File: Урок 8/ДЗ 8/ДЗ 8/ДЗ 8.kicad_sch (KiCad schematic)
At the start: 34 parts, among them K1 HONGFA_HFD2-0xx-x-L2-x, K2 HONGFA_HFD2-0xx-x-L2-x, SW1 SW_Push, SW2 SW_Push

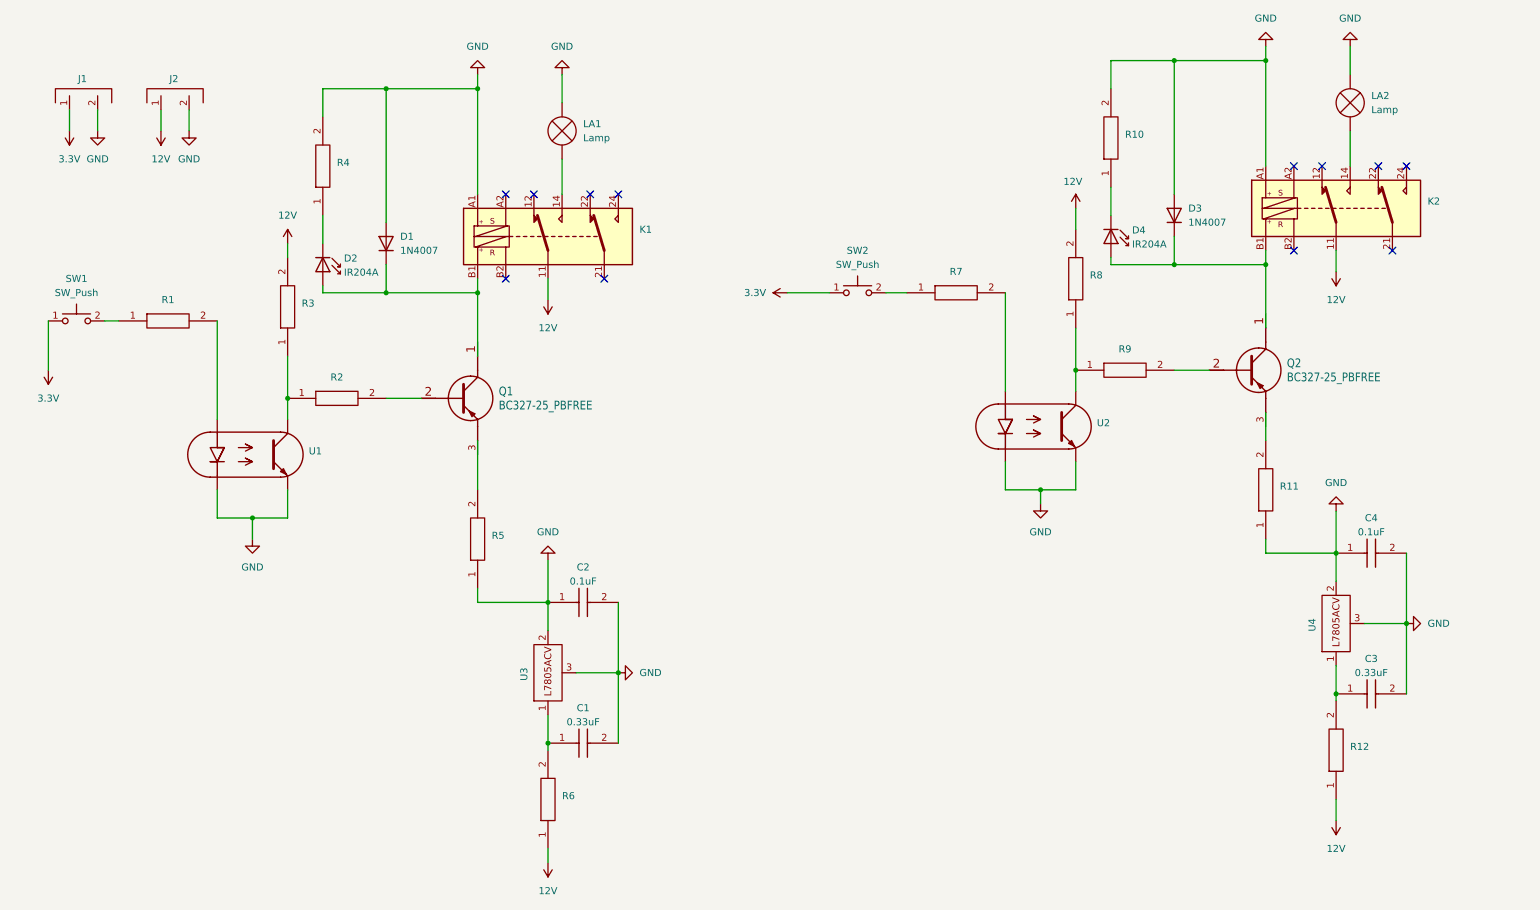
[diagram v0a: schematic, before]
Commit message: 1
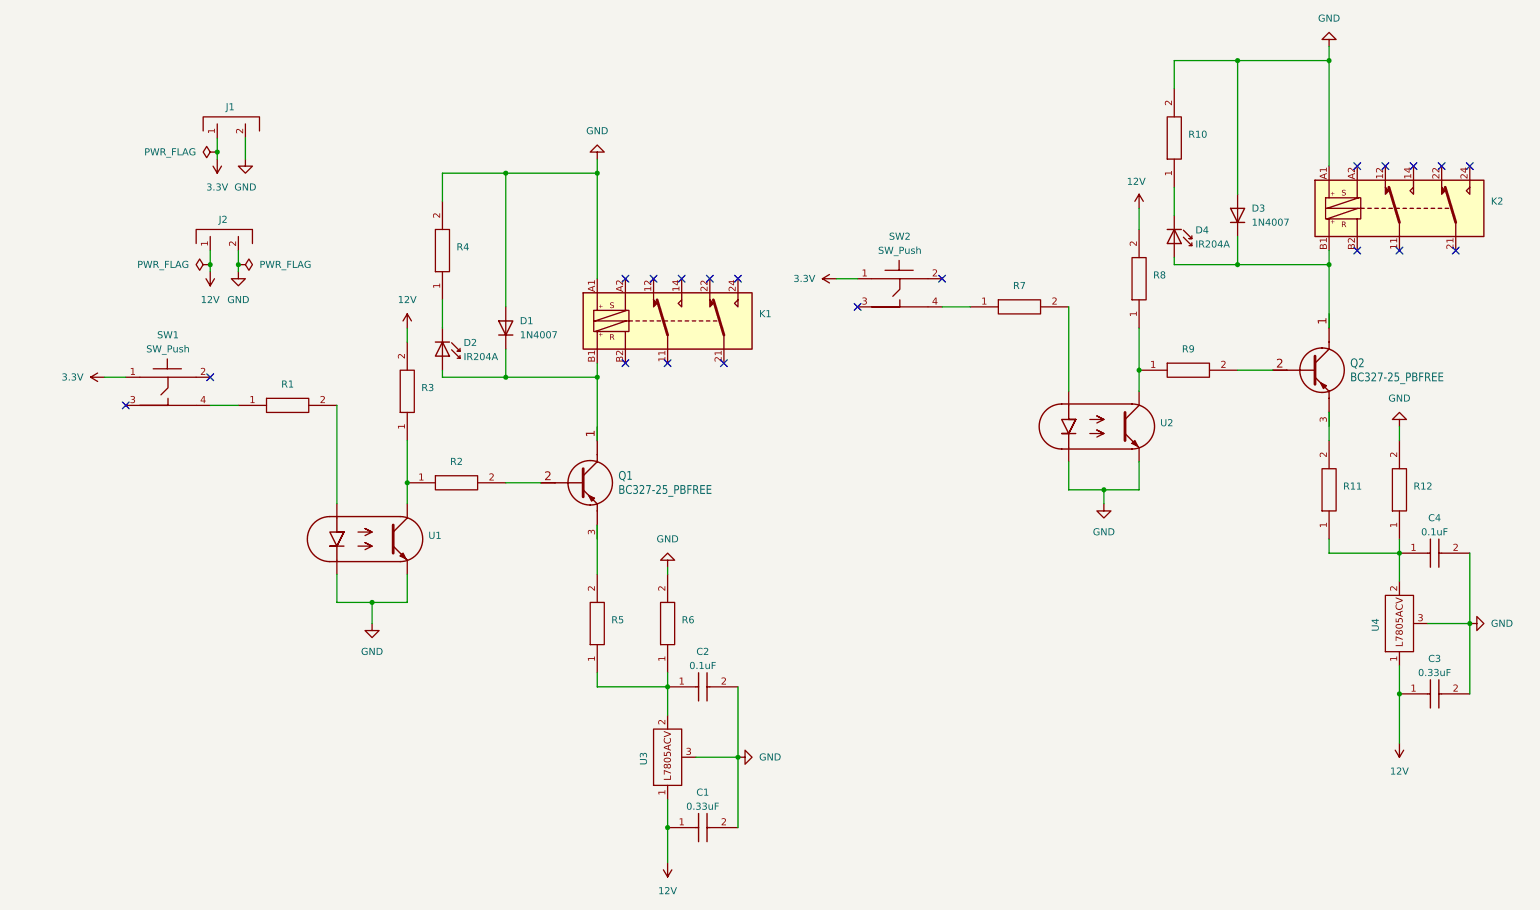
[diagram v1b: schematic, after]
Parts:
- removed LA1, LA2: Lamp, symbol Device:Lamp
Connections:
- net 12V: now also C1.1, C3.1, U3.1, U4.1; no longer K1.11, K2.11, R12.1, R6.1
- net GND: now also R12.2, R6.2; no longer C2.1, C4.1, R11.1, R5.1, U3.2, U4.2
- net at R1.1: now also SW1.4 (2); no longer SW1.2
- net at R7.1: now also SW2.4 (2); no longer SW2.2
- new net: C4.1, R11.1, R12.1, U4.2
- new net: C2.1, R5.1, R6.1, U3.2
- no-connect marks 12 -> 20
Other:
- moved on the sheet: C1, C2, C3, C4, D1, D2, D3, D4, J1, J2, K1, K2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

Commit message: 1
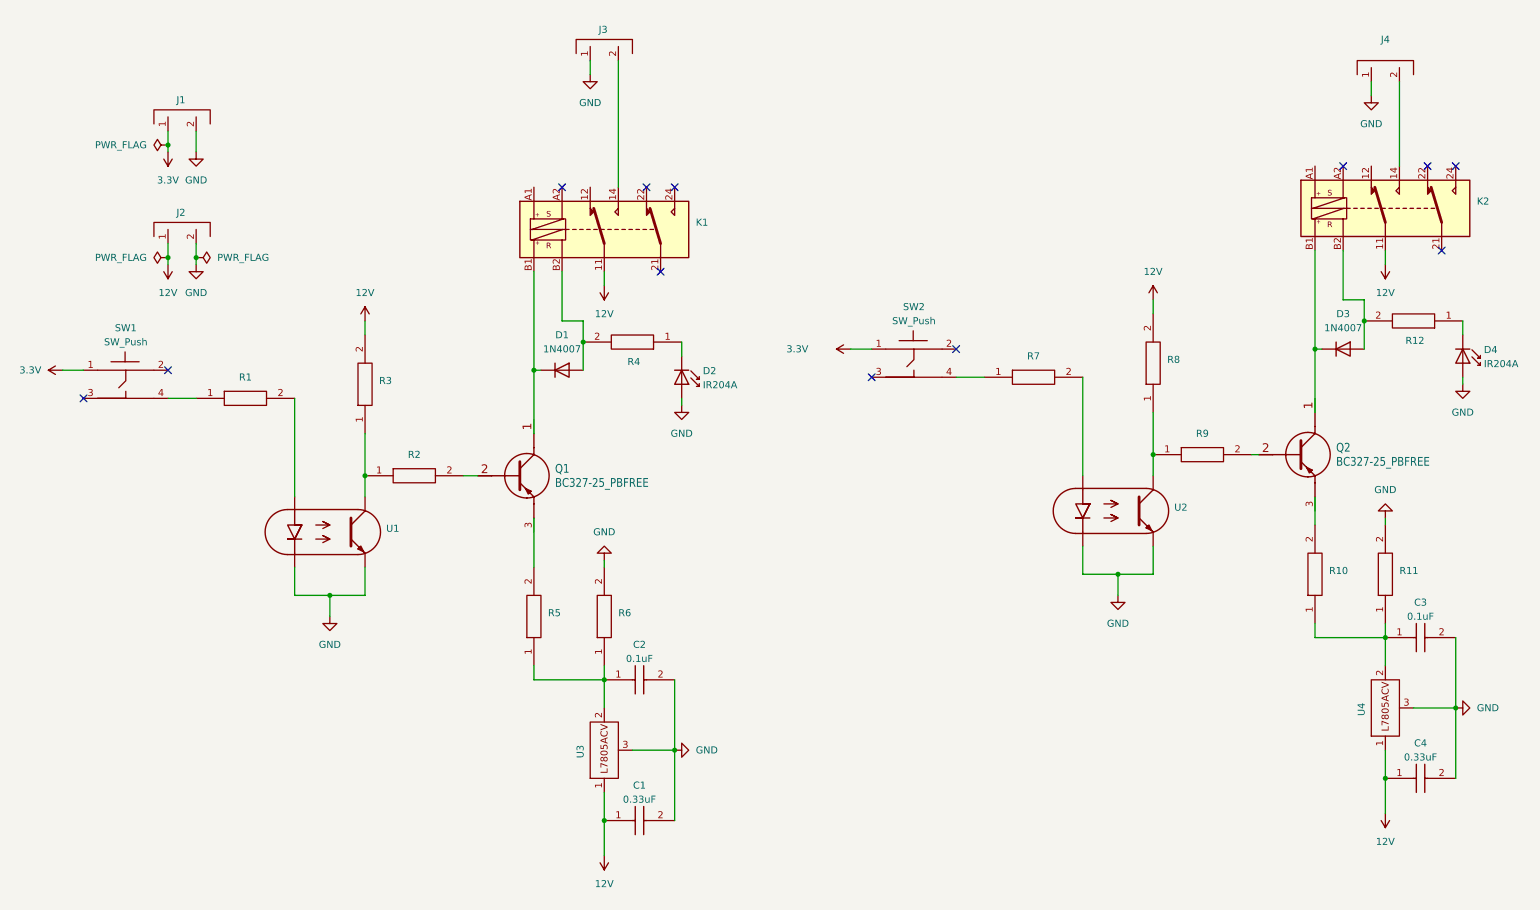
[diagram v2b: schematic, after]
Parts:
- added J3, J4: ~, My_lib2:TB-09A, symbol My_lib2:TB-09A
- C3: value 0.33uF -> 0.1uF
- C4: value 0.1uF -> 0.33uF
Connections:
- net 12V: now also C4.1, K1.11, K2.11; no longer C3.1
- net GND: now also D2.2 (A), D4.2 (A), R11.2, J3.1, J4.1; no longer D1.2 (A), D3.2 (A), K1.A1, K2.A1, R10.2, R12.2, R4.2
- net at R11.1, U4.2: now also C3.1, R10.1; no longer C4.1, R12.1
- net at D1.1 (K), K1.B1, Q1.1 (C): no longer D2.2 (A)
- net at D3.1 (K), K2.B1, Q2.1 (C): no longer D4.2 (A)
- net at Q2.3 (A): now also R10.2; no longer R11.2
- net at D4.1 (K): now also R12.1; no longer R10.1
- net at K2.14: now also J4.2
- net at K2.B2: now also D3.2 (A), R12.2
- net at K1.14: now also J3.2
- net at K1.B2: now also D1.2 (A), R4.2
- no-connect marks 20 -> 12
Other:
- moved on the sheet: C1, C2, D1, D2, J1, J2, K1, Q1, R1, R2, R3, R4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
